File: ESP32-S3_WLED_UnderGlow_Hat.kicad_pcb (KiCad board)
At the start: 6 copper layers, 31 x 29.2 mm, 142 parts, among them CN301 SM32B-NSHDZS-1-TF, CN302 SM32B-NSHDZS-1-TF, Q901 NTLJS17D0P03P8Z, U701 TCAN4550-Q1, U702 74LV1T125, U801 74LV1T125, U802 74LV1T125, U803 74LV1T125, U804 74LV1T125, U805 74LV1T125, U806 PCM1808, U901 74LV1T125, U902 74LV1T125, U903 TPS2HCS10A-Q1, U904 74LV1T125, U905 74LV1T125, U906 74LV1T125, U907 74LV1T125, Y701 40MHz

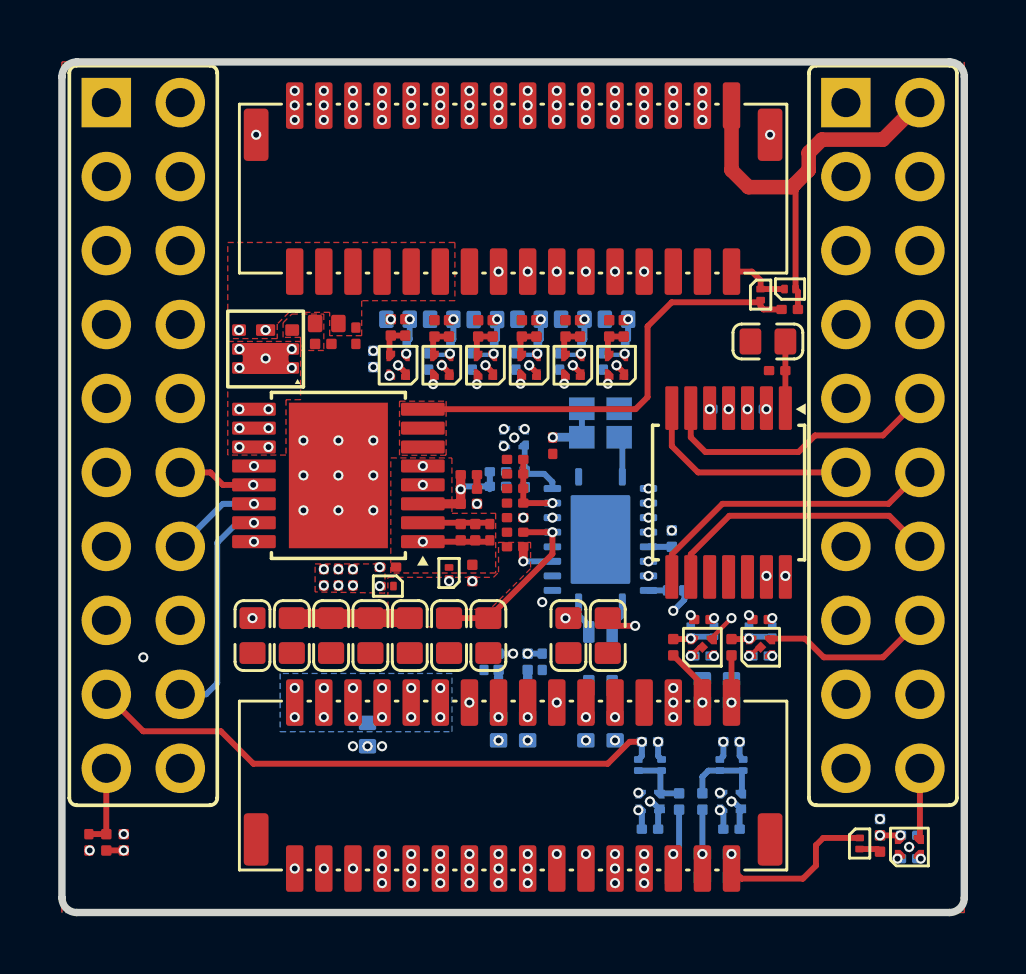
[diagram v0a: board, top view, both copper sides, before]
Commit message: Update .gitignore, CANBus_Interface.kicad_sch, ESP32-S3_WLED_UnderGlow_Hat-2026-05-04_233126.zip, and 17 more files
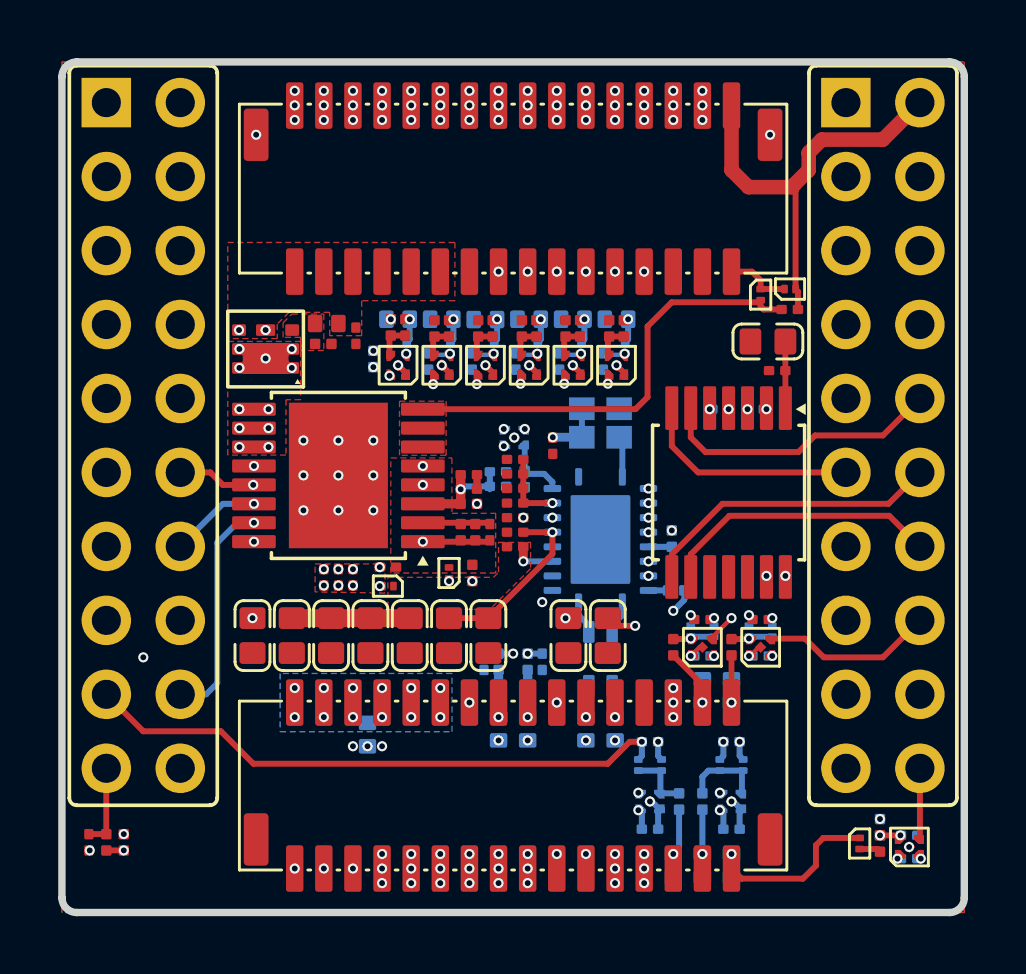
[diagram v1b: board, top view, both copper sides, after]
